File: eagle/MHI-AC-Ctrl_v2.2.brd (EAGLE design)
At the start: 59.9 x 31.7 mm, 25 parts, among them U1 TSR_1-2450

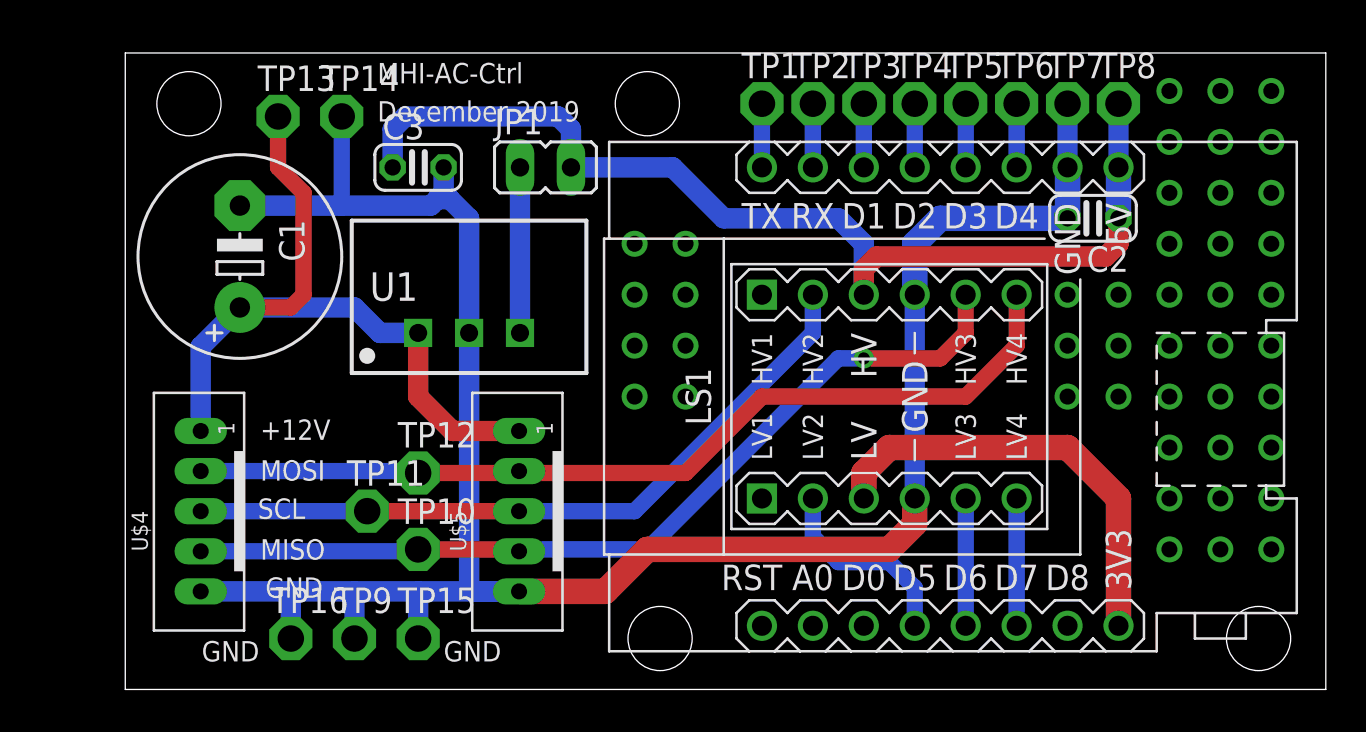
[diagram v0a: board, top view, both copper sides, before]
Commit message: PCB layout update
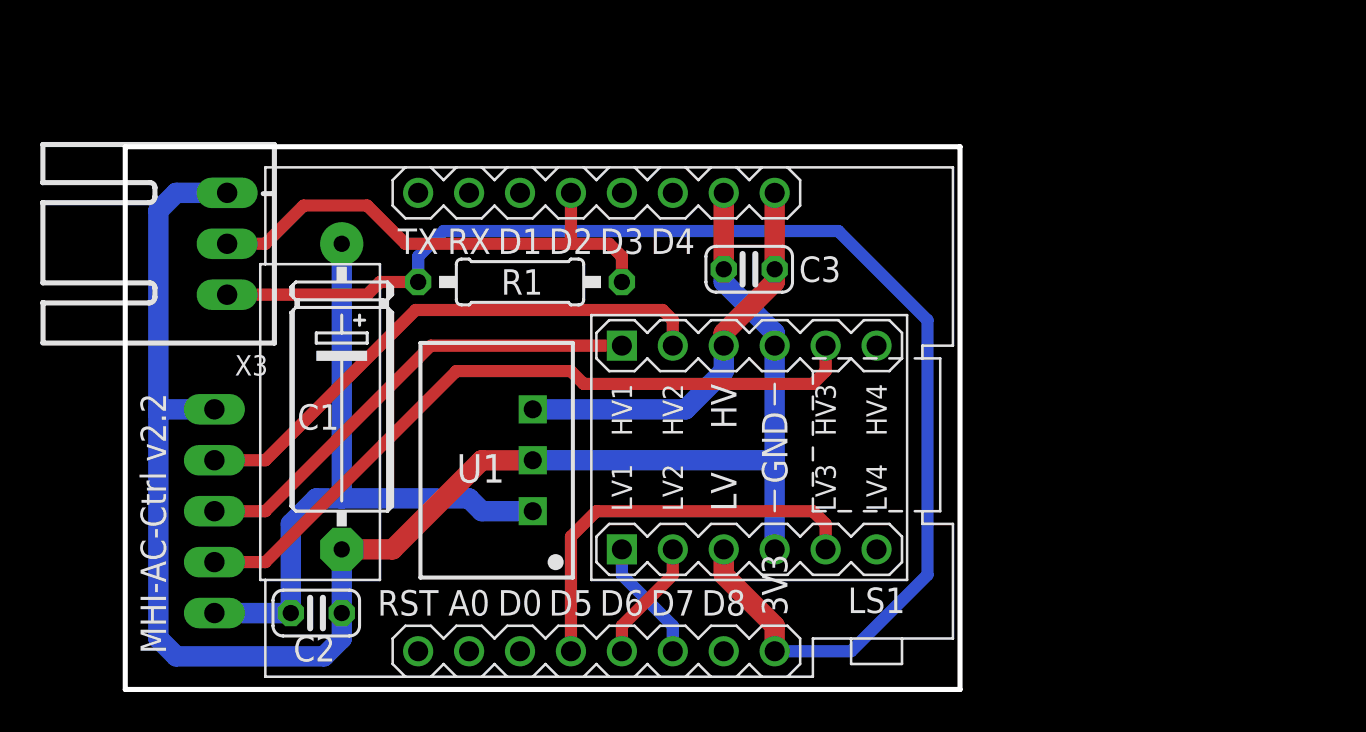
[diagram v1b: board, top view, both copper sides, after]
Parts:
- removed JP1: (no value), jumper:JP1
- removed TP1, TP10, TP11, TP12, TP13, TP14, TP15, TP16, TP2, TP3, TP4, TP5, TP6, TP7, TP8, TP9: TPPAD1-13, testpad:P1-13
- removed U$4, U$5: JST-PH_5-PIN_HEADER, srg:JST_B5B-PH_HEADER
- added R1: 4k7, rcl:0207/10
- added X1: JST 03JQ-BT, Rembrandt Electronics - JST XH Connectors v1-0:JST-XH-05-PACKAGE-LONG-PAD
- added X3: JST-XH-03-PIN, Rembrandt Electronics - JST XH Connectors v1-0:JST-XH-03-ST90-PACKAGE-LONG-PAD
- C1: value 22µ/50V -> 22µ/25V; device rcl:E5-10,5 -> rcl:E15-5
- C3: value 22p -> 100n
- moved C2 43.4 mm to (9.53, 3.81), turned to 0 degrees
- moved C3 17.3 mm to (31.1, 21.0), turned to 180 degrees
- moved U$1 17.2 mm to (24.1, 13.3)
- moved C1 8.64 mm to (10.8, 14.6), turned to 270 degrees
- moved LS1 7.43 mm to (31.1, 12.1)
- moved U1 7.10 mm to (20.3, 11.4), turned to 90 degrees
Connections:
- removed net N$10: TP2.TP, U$1.JP2.2
- removed net N$11: TP3.TP, U$1.JP2.3
- removed net N$12: TP4.TP, U$1.JP2.4
- removed net N$13: TP5.TP, U$1.JP2.5
- removed net N$14: TP6.TP, U$1.JP2.6
- removed net N$86: JP1.1, U1.3
- removed net N$9: TP1.TP, U$1.JP2.1
- removed net SCL: LS1.J2.2, TP11.TP, U$4.P3, U$5.P3
- removed net SCL_LV: LS1.J1.2, U$1.JP1.4
- new net D2: R1.2, U$1.JP2.4, X3.2
- new net SCK: LS1.J2.5, X1.4
- new net SCK_LV: LS1.J1.5, U$1.JP1.4
- net +12V: now also C2.1, X1.5; no longer TP13.TP, U$4.P1, U$5.P1
- net +3V3: now also R1.1, X3.1
- net +5V: now also U1.3; no longer C2.1, JP1.2, TP8.TP
- net GND: now also X1.1, X3.3; no longer TP14.TP, TP15.TP, TP16.TP, TP7.TP, TP9.TP, U$4.P5, U$5.P5
- net MISO: now also LS1.J2.2, X1.2; no longer LS1.J2.5, TP10.TP, U$4.P4, U$5.P4
- net MISO_LV: now also LS1.J1.2; no longer LS1.J1.5
- net MOSI: now also LS1.J2.1, X1.3; no longer LS1.J2.6, TP12.TP, U$4.P2, U$5.P2
- net MOSI_LV: now also LS1.J1.1; no longer LS1.J1.6
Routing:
- net +3V3: track 21.9 -> 66.9 mm
- net SCK: track 0.00 -> 36.2 mm
- net SCL: track 36.1 -> 0.00 mm
- net +5V: track 53.4 -> 20.3 mm
- net GND: track 111.0 -> 84.6 mm
- net D2: track 0.00 -> 25.3 mm
- net MOSI: track 46.1 -> 23.7 mm
- net SCK_LV: track 0.00 -> 20.5 mm
- net MISO: track 44.6 -> 27.4 mm, vias 1 -> 0
- net SCL_LV: track 9.94 -> 0.00 mm
- net N$86: track 8.25 -> 0.00 mm
- net +12V: track 38.2 -> 33.8 mm
- net N$9: track 3.18 -> 0.00 mm
- net N$14: track 3.18 -> 0.00 mm
- net N$13: track 3.18 -> 0.00 mm
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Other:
- board size 59.9 x 31.7 mm -> 41.6 x 27.1 mm
- board text added: "January 2021"
- board text added: "MHI-AC-Ctrl v2.2"
- board text removed: "+12V"
- board text removed: "December 2019"
- board text removed: "GND"
- board text removed: "MHI-AC-Ctrl"
- board text removed: "MISO"
- board text removed: "MOSI"
- board text removed: "SCL"
